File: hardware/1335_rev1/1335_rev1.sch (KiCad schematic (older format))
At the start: 20 parts, among them J1 Screw_Terminal_01x05, J2 Screw_Terminal_01x06, U1 A1335

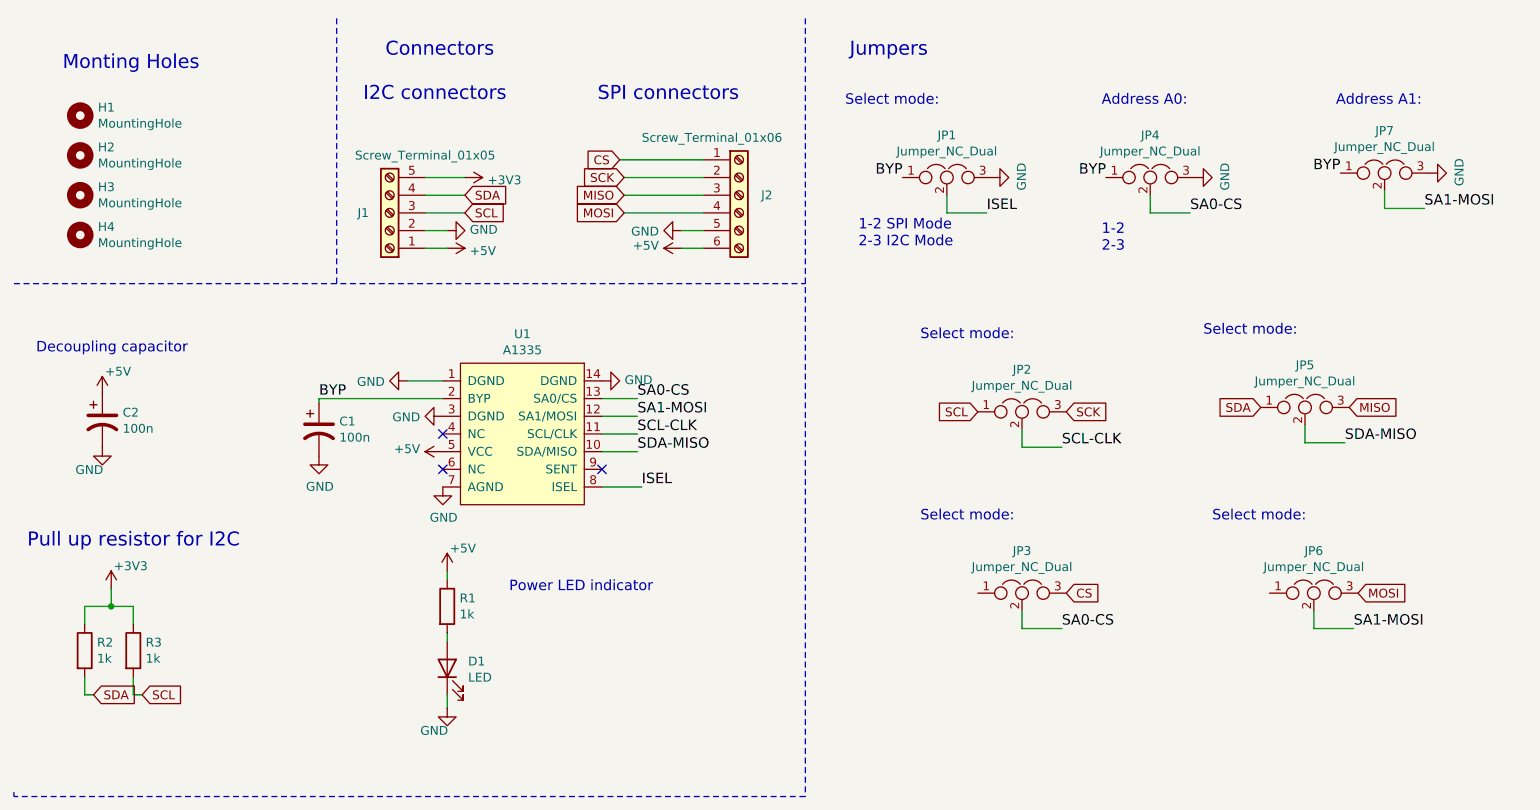
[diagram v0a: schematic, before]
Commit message: Send to review
Esteban Osella aprueba el diseño del PCB
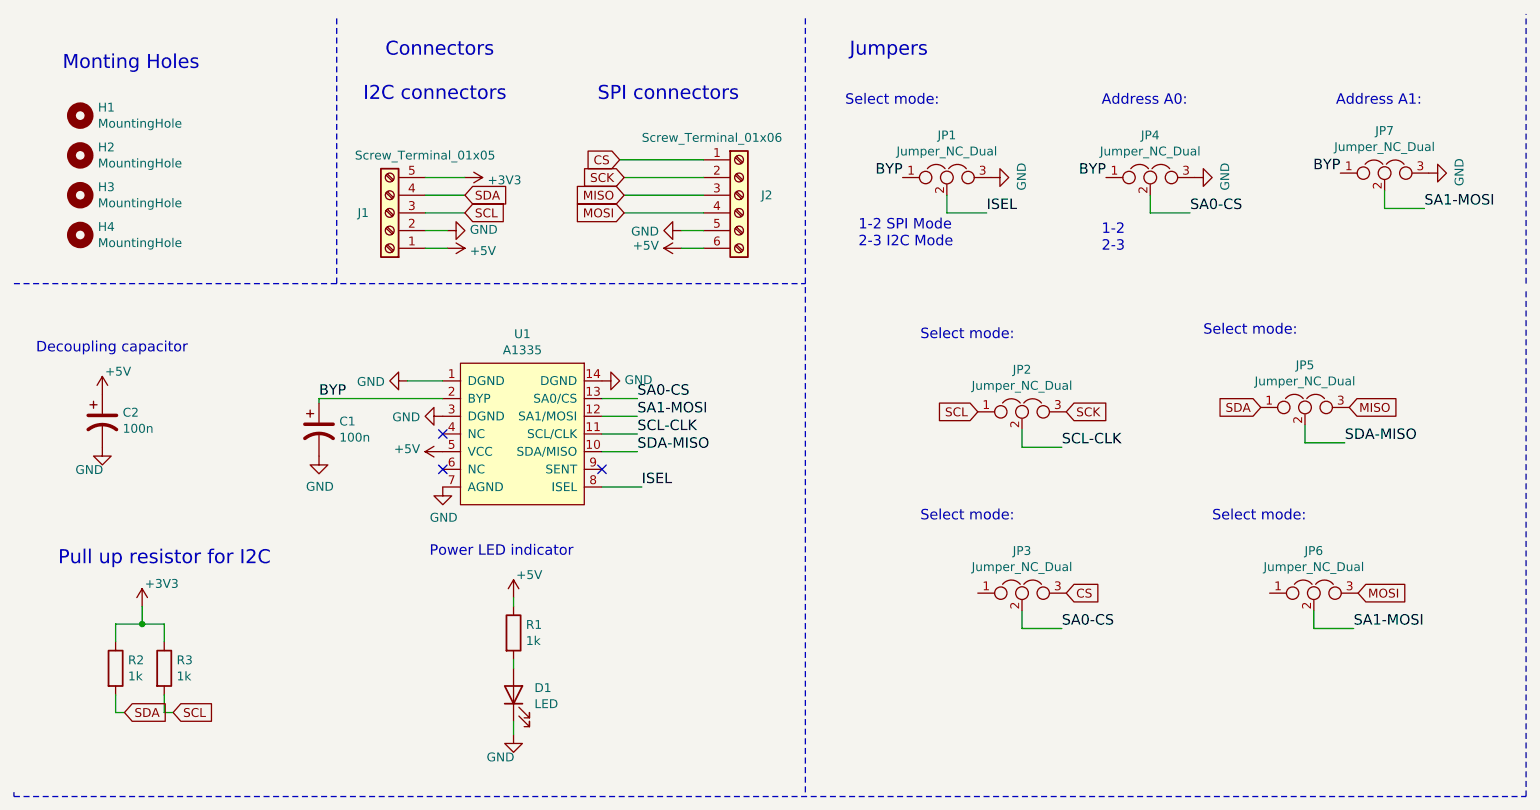
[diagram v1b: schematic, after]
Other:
- moved on the sheet: D1, R1, R2, R3
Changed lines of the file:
@@
 $Descr A4 11693 8268
 encoding utf-8
-Sheet 1 1
+Sheet 1 2
 Title "A1335 Allegro Sensor Board"
 Date "2021-03-29"
@@
 L power:+5V #PWR0116
 U 1 1 6047ABD4
-P 2975 3625
-F 0 "#PWR0116" H 2975 3475 50  0001 C CNN
-F 1 "+5V" H 2990 3753 50  0000 L CNN
-F 2 "" H 2975 3625 50  0001 C CNN
-F 3 "" H 2975 3625 50  0001 C CNN
-	1    2975 3625
+P 3350 3775
+F 0 "#PWR0116" H 3350 3625 50  0001 C CNN
+F 1 "+5V" H 3365 3903 50  0000 L CNN
+F 2 "" H 3350 3775 50  0001 C CNN
+F 3 "" H 3350 3775 50  0001 C CNN
+	1    3350 3775
 	1    0    0    -1
 $EndComp
@@
 L power:GND #PWR0117
 U 1 1 6047B169
-P 2975 4400
-F 0 "#PWR0117" H 2975 4150 50  0001 C CNN
-F 1 "GND" H 2980 4272 50  0000 R CNN
-F 2 "" H 2975 4400 50  0001 C CNN
-F 3 "" H 2975 4400 50  0001 C CNN
-	1    2975 4400
+P 3350 4550
+F 0 "#PWR0117" H 3350 4300 50  0001 C CNN
+F 1 "GND" H 3355 4422 50  0000 R CNN
+F 2 "" H 3350 4550 50  0001 C CNN
+F 3 "" H 3350 4550 50  0001 C CNN
+	1    3350 4550
 	1    0    0    -1
 $EndComp
@@
 L Device:LED D1
 U 1 1 6047BFDB
-P 2975 4175
-F 0 "D1" V 3014 4057 50  0000 R CNN
-F 1 "LED" V 2923 4057 50  0000 R CNN
-F 2 "LED_SMD:LED_0603_1608Metric" H 2975 4175 50  0001 C CNN
-F 3 "~" H 2975 4175 50  0001 C CNN
-	1    2975 4175
+P 3350 4325
+F 0 "D1" V 3389 4207 50  0000 R CNN
+F 1 "LED" V 3298 4207 50  0000 R CNN
+F 2 "LED_SMD:LED_0603_1608Metric" H 3350 4325 50  0001 C CNN
+F 3 "~" H 3350 4325 50  0001 C CNN
+	1    3350 4325
 	0    -1   -1   0
 $EndComp
@@
 L Device:R R1
 U 1 1 6047CC80
-P 2975 3825
-F 0 "R1" H 3045 3871 50  0000 L CNN
-F 1 "1k" H 3045 3780 50  0000 L CNN
-F 2 "Resistor_SMD:R_0603_1608Metric" V 2905 3825 50  0001 C CNN
-F 3 "~" H 2975 3825 50  0001 C CNN
-	1    2975 3825
-	1    0    0    -1
-$EndComp
-Wire Wire Line
-	2975 3675 2975 3625
-Wire Wire Line
-	2975 3975 2975 4025
-Wire Wire Line
-	2975 4400 2975 4325
+P 3350 3975
+F 0 "R1" H 3420 4021 50  0000 L CNN
+F 1 "1k" H 3420 3930 50  0000 L CNN
+F 2 "Resistor_SMD:R_0603_1608Metric" V 3280 3975 50  0001 C CNN
+F 3 "~" H 3350 3975 50  0001 C CNN
+	1    3350 3975
+	1    0    0    -1
+$EndComp
+Wire Wire Line
+	3350 3825 3350 3775
+Wire Wire Line
+	3350 4125 3350 4175
+Wire Wire Line
+	3350 4550 3350 4475
 $Comp
 L Device:R R3
 U 1 1 604B0FB7
-P 1200 4075
-F 0 "R3" H 1270 4121 50  0000 L CNN
-F 1 "1k" H 1270 4030 50  0000 L CNN
-F 2 "Resistor_SMD:R_0603_1608Metric" V 1130 4075 50  0001 C CNN
-F 3 "~" H 1200 4075 50  0001 C CNN
-	1    1200 4075
+P 1375 4175
+F 0 "R3" H 1445 4221 50  0000 L CNN
+F 1 "1k" H 1445 4130 50  0000 L CNN
+F 2 "Resistor_SMD:R_0603_1608Metric" V 1305 4175 50  0001 C CNN
+F 3 "~" H 1375 4175 50  0001 C CNN
+	1    1375 4175
 	1    0    0    -1
 $EndComp
@@
 L Device:R R2
 U 1 1 604B1BBC
-P 925 4075
-F 0 "R2" H 995 4121 50  0000 L CNN
-F 1 "1k" H 995 4030 50  0000 L CNN
-F 2 "Resistor_SMD:R_0603_1608Metric" V 855 4075 50  0001 C CNN
-F 3 "~" H 925 4075 50  0001 C CNN
-	1    925  4075
+P 1100 4175
+F 0 "R2" H 1170 4221 50  0000 L CNN
+F 1 "1k" H 1170 4130 50  0000 L CNN
+F 2 "Resistor_SMD:R_0603_1608Metric" V 1030 4175 50  0001 C CNN
+F 3 "~" H 1100 4175 50  0001 C CNN
+	1    1100 4175
 	1    0    0    -1
 $EndComp
@@
 	3950 1300 4425 1300
 Wire Wire Line
-	925  4225 925  4325
-Wire Wire Line
-	1200 4225 1200 4325
-Wire Wire Line
-	925  3925 925  3825
-Wire Wire Line
-	925  3825 1075 3825
-Wire Wire Line
-	1200 3825 1200 3925
-Connection ~ 1075 3825
-Wire Wire Line
-	1075 3825 1200 3825
+	1100 4325 1100 4425
+Wire Wire Line
+	1375 4325 1375 4425
+Wire Wire Line
+	1100 4025 1100 3925
+Wire Wire Line
+	1100 3925 1250 3925
+Wire Wire Line
+	1375 3925 1375 4025
+Connection ~ 1250 3925
+Wire Wire Line
+	1250 3925 1375 3925
 $Comp
 L power:+3V3 #PWR0118
 U 1 1 604BB954
-P 1075 3725
-F 0 "#PWR0118" H 1075 3575 50  0001 C CNN
-F 1 "+3V3" H 1090 3853 50  0000 L CNN
-F 2 "" H 1075 3725 50  0001 C CNN
-F 3 "" H 1075 3725 50  0001 C CNN
-	1    1075 3725
+P 1250 3825
+F 0 "#PWR0118" H 1250 3675 50  0001 C CNN
+F 1 "+3V3" H 1265 3953 50  0000 L CNN
+F 2 "" H 1250 3825 50  0001 C CNN
+F 3 "" H 1250 3825 50  0001 C CNN
+	1    1250 3825
 	1    0    0    -1
 $EndComp
@@
 Text Notes 3825 975  0    79   ~ 0
 SPI connectors
-Text GLabel 975  4325 2    50   Input ~ 0
+Text GLabel 1150 4425 2    50   Input ~ 0
 SDA
-Text GLabel 1250 4325 2    50   Input ~ 0
+Text GLabel 1425 4425 2    50   Input ~ 0
 SCL
 Wire Wire Line
-	1250 4325 1200 4325
-Wire Wire Line
-	975  4325 925  4325
-Wire Wire Line
-	1075 3825 1075 3725
+	1425 4425 1375 4425
+Wire Wire Line
+	1150 4425 1100 4425
+Wire Wire Line
+	1250 3925 1250 3825
 $Comp
 L Connector:Screw_Terminal_01x05 J1
@@
 NoConn ~ 3850 3050
 Wire Notes Line
-	5000 4900 525  4900
-Wire Notes Line
 	525  4900 525  4875
 Wire Notes Line
@@
 Text Notes 6675 1825 0    59   ~ 0
 1-2\n2-3
-Text Notes 600  3500 0    79   ~ 0
+Text Notes 775  3600 0    79   ~ 0
 Pull up resistor for I2C
-Text Notes 3325 3750 0    59   ~ 0
+Text Notes 2875 3550 0    59   ~ 0
 Power LED indicator
+Wire Notes Line
+	9075 4900 9075 2025
+Wire Notes Line
+	525  4900 9075 4900
+Wire Notes Line
+	9075 2000 9075 475
 $EndSCHEMATC

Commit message: Error in boom
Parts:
- C1, C2: footprint Capacitor_Tantalum_SMD:CP_EIA-1608-08_AVX-J -> Capacitor_Tantalum_SMD:CP_EIA-2012-15_AVX-P_Pad1.30x1.05mm_HandSolder
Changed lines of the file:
@@
 $Descr A4 11693 8268
 encoding utf-8
-Sheet 1 2
+Sheet 1 1
 Title "A1335 Allegro Sensor Board"
 Date "2021-03-29"
@@
 F 0 "C1" H 2365 2871 50  0000 L CNN
 F 1 "100n" H 2365 2780 50  0000 L CNN
-F 2 "Capacitor_Tantalum_SMD:CP_EIA-1608-08_AVX-J" H 2250 2825 50  0001 C CNN
+F 2 "Capacitor_Tantalum_SMD:CP_EIA-2012-15_AVX-P_Pad1.30x1.05mm_HandSolder" H 2250 2825 50  0001 C CNN
 F 3 "~" H 2250 2825 50  0001 C CNN
 	1    2250 2825
@@
 F 0 "C2" H 1140 2821 50  0000 L CNN
 F 1 "100n" H 1140 2730 50  0000 L CNN
-F 2 "Capacitor_Tantalum_SMD:CP_EIA-1608-08_AVX-J" H 1025 2775 50  0001 C CNN
+F 2 "Capacitor_Tantalum_SMD:CP_EIA-2012-15_AVX-P_Pad1.30x1.05mm_HandSolder" H 1025 2775 50  0001 C CNN
 F 3 "~" H 1025 2775 50  0001 C CNN
 	1    1025 2775
